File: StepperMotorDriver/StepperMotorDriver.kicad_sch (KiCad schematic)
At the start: 1 part, among them U1 A4988SETTR-T

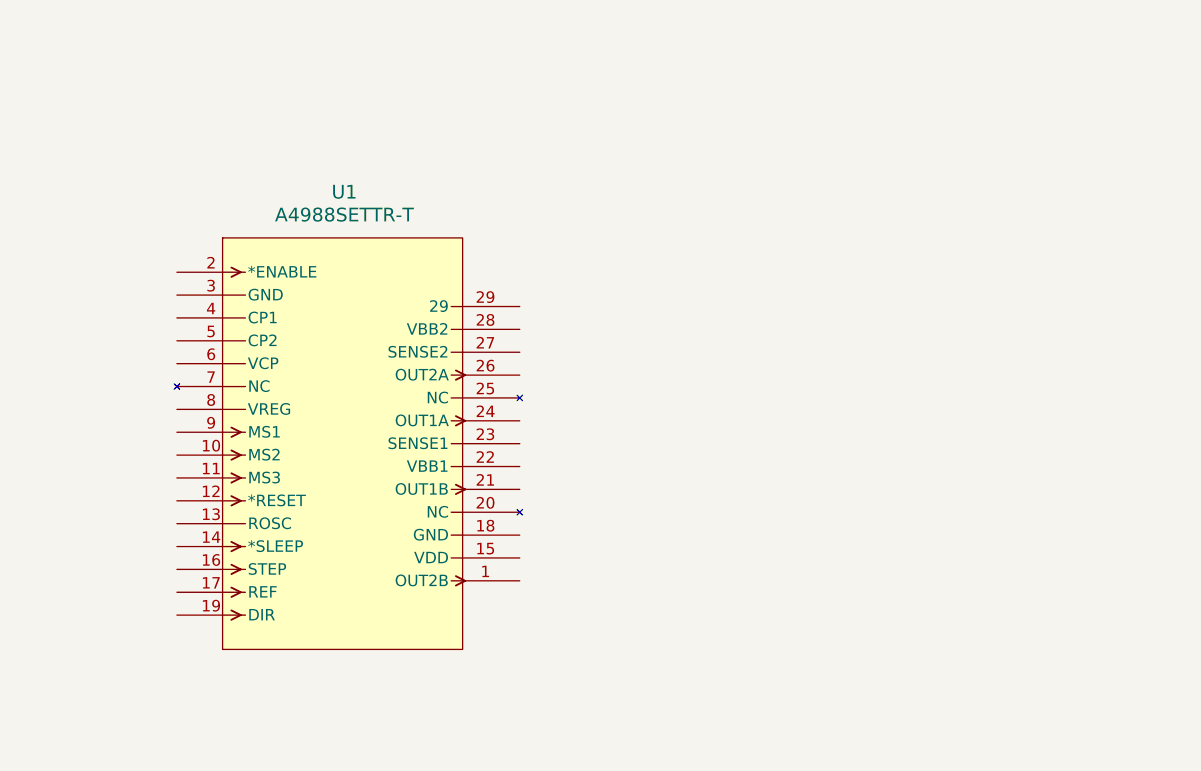
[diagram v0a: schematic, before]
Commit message: edited schematic
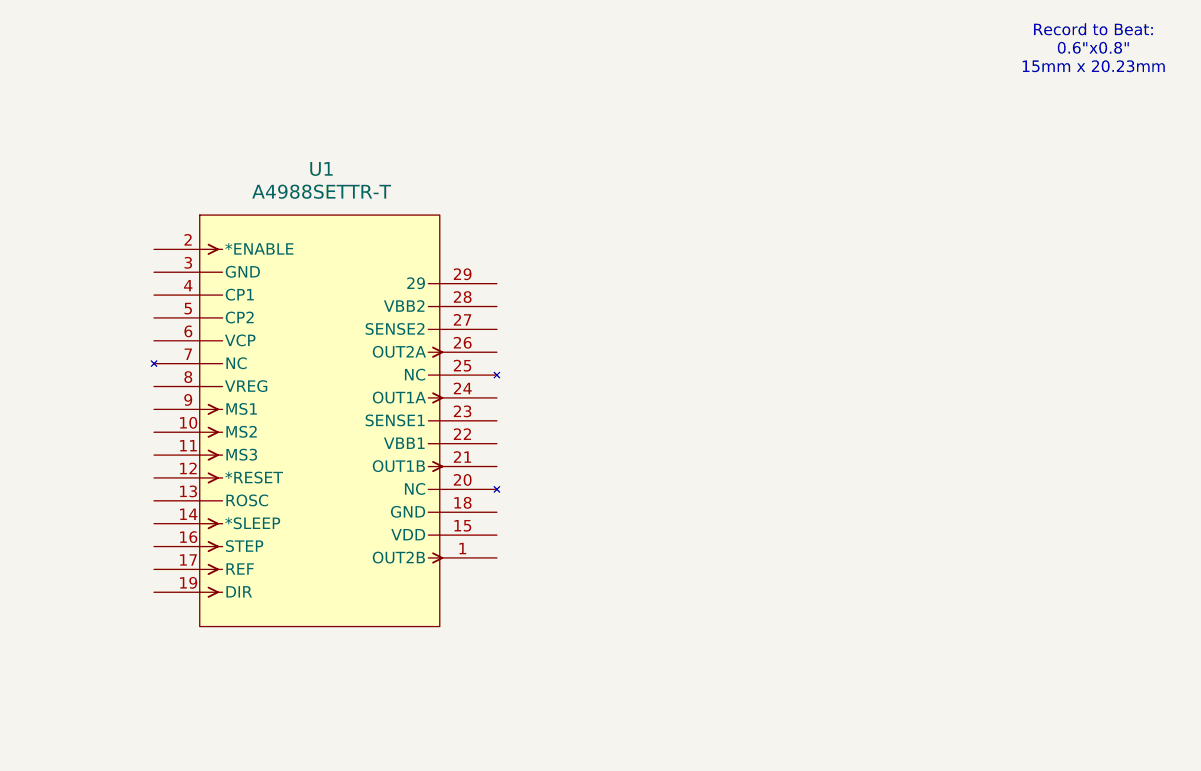
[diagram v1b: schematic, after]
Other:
- note added: "Record to Beat: 0.6"x0.8" 15mm x 20.23mm"
- moved on the sheet: U1
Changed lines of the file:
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@@
 	(generator_version "8.0")
 	(paper "A5")
+	(text "Record to Beat: \n0.6\"x0.8\"\n15mm x 20.23mm"
+		(exclude_from_sim no)
+		(at 185.674 19.812 0)
+		(effects
+			(font
+				(size 1.27 1.27)
+			)
+		)
+	)
 	(symbol
 		(lib_id "Project_Symbols:A4988SETTR-T")
-		(at 83.82 44.45 0)
+		(at 81.28 41.91 0)
 		(unit 1)
 		(exclude_from_sim no)
@@
 		(fields_autoplaced yes)
 		(property "Reference" "U1"
-			(at 102.4318 35.56 0)
+			(at 99.8918 33.02 0)
 			(effects
 				(font
@@
 		)
 		(property "Value" "A4988SETTR-T"
-			(at 102.4318 38.1 0)
+			(at 99.8918 35.56 0)
 			(effects
 				(font
@@
 		)
 		(property "Footprint" "QFN-28_ALM"
-			(at 101.6 41.91 0)
+			(at 99.06 39.37 0)
 			(effects
 				(font
@@
 		)
 		(property "Datasheet" "A4988SETTR-T"
-			(at 101.6 39.37 0)
+			(at 99.06 36.83 0)
 			(effects
 				(font
@@
 		)
 		(property "Description" ""
-			(at 83.82 44.45 0)
+			(at 81.28 41.91 0)
 			(effects
 				(font

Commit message: Edited Schematic
Changed main IC symbol
Added Peripheral components
Assigned footprints
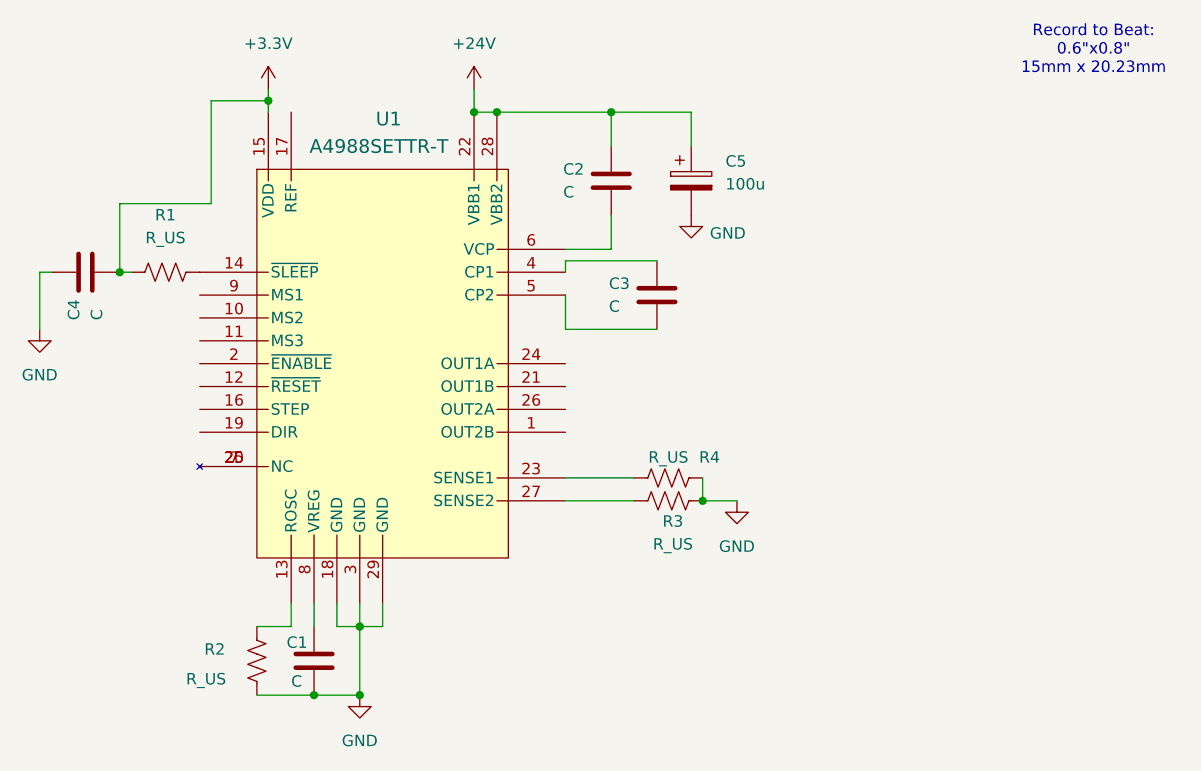
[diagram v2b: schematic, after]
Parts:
- added C1, C2, C3, C4: C, symbol Device:C
- added C5: 100u, symbol Device:C_Polarized
- added R1, R2, R3, R4: R_US, symbol Device:R_US
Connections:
- net at U1.13 (ROSC): now also R2.2
- net at U1.14 (~{SLEEP}): now also R1.2
- net +3.3V: now reaches U1.15 (VDD)
- net +3.3V: now also C4.1, R1.1
- net GND: now reaches U1.18 (GND)
- net GND: now also U1.29 (GND), U1.3 (GND), C1.1, C4.2, C5.2, R2.1, R3.2, R4.2
- net at U1.20 (NC): now also U1.25 (NC), U1.7 (NC)
- net +24V: now reaches U1.22 (VBB1)
- net +24V: now also U1.28 (VBB2), C2.2, C5.1
- net at U1.23 (SENSE1): now also R4.1
- net at U1.27 (SENSE2): now also R3.1
- net at U1.4 (CP1): now also C3.2
- net at U1.5 (CP2): now also C3.1
- net at U1.6 (VCP): now also C2.1
- net at U1.8 (VREG): now also C1.2
